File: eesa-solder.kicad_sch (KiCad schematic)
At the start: 5 parts

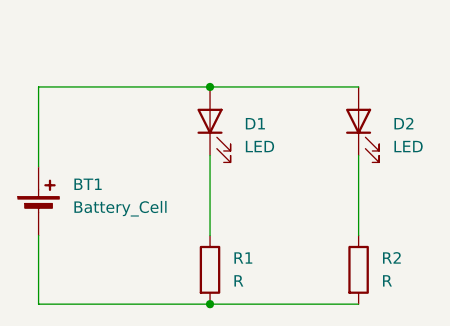
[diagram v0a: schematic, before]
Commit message: push to github
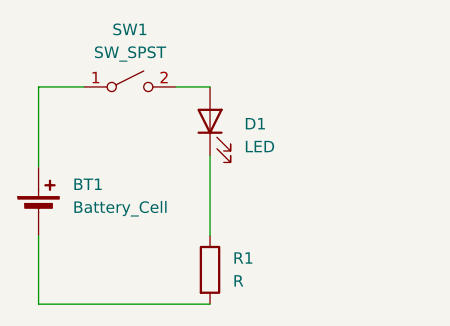
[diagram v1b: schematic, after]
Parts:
- removed D2: LED, LED_THT:LED_D5.0mm, symbol Device:LED
- removed R2: R, Resistor_THT:R_Axial_DIN0207_L6.3mm_D2.5mm_P7.62mm_Horizontal, symbol Device:R
- added SW1: SW_SPST, Button_Switch_THT:SW_Slide_SPDT_Straight_CK_OS102011MS2Q, symbol Switch:SW_SPST
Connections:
- net at D1.2 (A): now also SW1.2 (B); no longer BT1.1 (+)
- new net: BT1.1 (+), SW1.1 (A)
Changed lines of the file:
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@@
 	(generator_version "9.0")
 	(paper "A4")
-	(junction
-		(at 124.46 80.01)
-		(diameter 0)
-		(color 0 0 0 0)
-	)
-	(junction
-		(at 124.46 104.14)
-		(diameter 0)
-		(color 0 0 0 0)
-	)
 	(wire
 		(pts
@@
 	(wire
 		(pts
-			(xy 140.97 104.14) (xy 124.46 104.14)
+			(xy 124.46 104.14) (xy 105.41 104.14)
 		)
 		(stroke
@@
 	(wire
 		(pts
-			(xy 124.46 80.01) (xy 140.97 80.01)
+			(xy 105.41 80.01) (xy 110.49 80.01)
 		)
 		(stroke
@@
 	(wire
 		(pts
-			(xy 140.97 87.63) (xy 140.97 96.52)
-		)
-		(stroke
-			(width 0)
-			(type default)
-		)
-	)
-	(wire
-		(pts
-			(xy 105.41 80.01) (xy 124.46 80.01)
-		)
-		(stroke
-			(width 0)
-			(type default)
-		)
-	)
-	(wire
-		(pts
-			(xy 124.46 104.14) (xy 105.41 104.14)
+			(xy 120.65 80.01) (xy 124.46 80.01)
 		)
 		(stroke
@@
 			(width 0)
 			(type default)
-		)
-	)
-	(symbol
-		(lib_id "Device:LED")
-		(at 140.97 83.82 90)
-		(unit 1)
-		(exclude_from_sim no)
-		(in_bom yes)
-		(on_board yes)
-		(dnp no)
-		(fields_autoplaced yes)
-		(property "Reference" "D2"
-			(at 144.78 84.1374 90)
-			(effects
-				(font
-					(size 1.27 1.27)
-				)
-				(justify right)
-			)
-		)
-		(property "Value" "LED"
-			(at 144.78 86.6774 90)
-			(effects
-				(font
-					(size 1.27 1.27)
-				)
-				(justify right)
-			)
-		)
-		(property "Footprint" "LED_THT:LED_D5.0mm"
-			(at 140.97 83.82 0)
-			(effects
-				(font
-					(size 1.27 1.27)
-				)
-				(hide yes)
-			)
-		)
-		(property "Datasheet" "~"
-			(at 140.97 83.82 0)
-			(effects
-				(font
-					(size 1.27 1.27)
-				)
-				(hide yes)
-			)
-		)
-		(property "Description" "Light emitting diode"
-			(at 140.97 83.82 0)
-			(effects
-				(font
-					(size 1.27 1.27)
-				)
-				(hide yes)
-			)
-		)
-		(property "Sim.Pins" "1=K 2=A"
-			(at 140.97 83.82 0)
-			(effects
-				(font
-					(size 1.27 1.27)
-				)
-				(hide yes)
-			)
-		)
-		(pin "1"
-		)
-		(pin "2"
-		)
-		(instances
-			(project ""
-				(path "/d60e8bd7-a134-48bf-bf86-f755bbb52909"
-					(reference "D2")
-					(unit 1)
-				)
-			)
-		)
-	)
-	(symbol
-		(lib_id "Device:R")
-		(at 140.97 100.33 0)
-		(unit 1)
-		(exclude_from_sim no)
-		(in_bom yes)
-		(on_board yes)
-		(dnp no)
-		(fields_autoplaced yes)
-		(property "Reference" "R2"
-			(at 143.51 99.0599 0)
-			(effects
-				(font
-					(size 1.27 1.27)
-				)
-				(justify left)
-			)
-		)
-		(property "Value" "R"
-			(at 143.51 101.5999 0)
-			(effects
-				(font
-					(size 1.27 1.27)
-				)
-				(justify left)
-			)
-		)
-		(property "Footprint" "Resistor_THT:R_Axial_DIN0207_L6.3mm_D2.5mm_P7.62mm_Horizontal"
-			(at 139.192 100.33 90)
-			(effects
-				(font
-					(size 1.27 1.27)
-				)
-				(hide yes)
-			)
-		)
-		(property "Datasheet" "~"
-			(at 140.97 100.33 0)
-			(effects
-				(font
-					(size 1.27 1.27)
-				)
-				(hide yes)
-			)
-		)
-		(property "Description" "Resistor"
-			(at 140.97 100.33 0)
-			(effects
-				(font
-					(size 1.27 1.27)
-				)
-				(hide yes)
-			)
-		)
-		(pin "1"
-		)
-		(pin "2"
-		)
-		(instances
-			(project ""
-				(path "/d60e8bd7-a134-48bf-bf86-f755bbb52909"
-					(reference "R2")
-					(unit 1)
-				)
-			)
 		)
 	)
@@
 					(unit 1)
 				)
+			)
+		)
+	)
+	(symbol
+		(lib_id "Switch:SW_SPST")
+		(at 115.57 80.01 0)
+		(unit 1)
+		(exclude_from_sim no)
+		(in_bom yes)
+		(on_board yes)
+		(dnp no)
+		(fields_autoplaced yes)
+		(property "Reference" "SW1"
+			(at 115.57 73.66 0)
+			(effects
+				(font
+					(size 1.27 1.27)
+				)
+			)
+		)
+		(property "Value" "SW_SPST"
+			(at 115.57 76.2 0)
+			(effects
+				(font
+					(size 1.27 1.27)
+				)
+			)
+		)
+		(property "Footprint" "Button_Switch_THT:SW_Slide_SPDT_Straight_CK_OS102011MS2Q"
+			(at 115.57 80.01 0)
+			(effects
+				(font
+					(size 1.27 1.27)
+				)
+				(hide yes)
+			)
+		)
+		(property "Datasheet" "~"
+			(at 115.57 80.01 0)
+			(effects
+				(font
+					(size 1.27 1.27)
+				)
+				(hide yes)
+			)
+		)
+		(property "Description" "Single Pole Single Throw (SPST) switch"
+			(at 115.57 80.01 0)
+			(effects
+				(font
+					(size 1.27 1.27)
+				)
+				(hide yes)
+			)
+		)
+		(pin "1"
+		)
+		(pin "2"
+		)
+		(instances
+			(project ""
+				(path "/d60e8bd7-a134-48bf-bf86-f755bbb52909"
+					(reference "SW1")
+					(unit 1)
+				)
